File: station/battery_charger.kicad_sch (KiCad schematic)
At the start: 1 part, among them J8 Conn_01x04

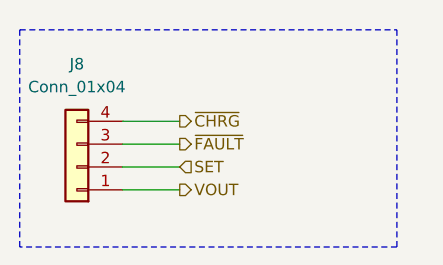
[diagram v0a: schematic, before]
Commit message: Signed-off-by: Scott Perkins <whatisbyandby@gmail.com>
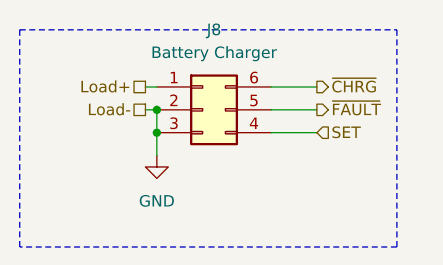
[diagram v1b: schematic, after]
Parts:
- removed J8: Conn_01x04, Connector_PinSocket_2.54mm:PinSocket_1x04_P2.54mm_Horizontal, symbol Connector_Generic:Conn_01x04
- added J8: Battery Charger, Connector_PinSocket_2.54mm:PinSocket_2x03_P2.54mm_Vertical, symbol Connector_Generic:Conn_02x03_Counter_Clockwise
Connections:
- net SET: now also J8.4 (Pin_4)
- net ~{CHRG}: now also J8.6 (Pin_6)
- net ~{FAULT}: now also J8.5 (Pin_5)
- new net GND: J8.2 (Pin_2), J8.3 (Pin_3)
- new net Load+: J8.1 (Pin_1)
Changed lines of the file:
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@@
 	(generator_version "8.0")
 	(paper "A4")
-	(wire
-		(pts
-			(xy 109.22 91.44) (xy 115.57 91.44)
-		)
-		(stroke
-			(width 0)
-			(type default)
-		)
-	)
-	(wire
-		(pts
-			(xy 109.22 86.36) (xy 115.57 86.36)
-		)
-		(stroke
-			(width 0)
-			(type default)
-		)
-	)
-	(wire
-		(pts
-			(xy 109.22 88.9) (xy 115.57 88.9)
-		)
-		(stroke
-			(width 0)
-			(type default)
-		)
-	)
-	(wire
-		(pts
-			(xy 109.22 93.98) (xy 115.57 93.98)
+	(junction
+		(at 113.03 87.63)
+		(diameter 0)
+		(color 0 0 0 0)
+	)
+	(junction
+		(at 113.03 85.09)
+		(diameter 0)
+		(color 0 0 0 0)
+	)
+	(wire
+		(pts
+			(xy 125.73 87.63) (xy 130.81 87.63)
+		)
+		(stroke
+			(width 0)
+			(type default)
+		)
+	)
+	(wire
+		(pts
+			(xy 113.03 87.63) (xy 113.03 90.17)
+		)
+		(stroke
+			(width 0)
+			(type default)
+		)
+	)
+	(wire
+		(pts
+			(xy 111.76 85.09) (xy 113.03 85.09)
+		)
+		(stroke
+			(width 0)
+			(type default)
+		)
+	)
+	(wire
+		(pts
+			(xy 125.73 82.55) (xy 130.81 82.55)
+		)
+		(stroke
+			(width 0)
+			(type default)
+		)
+	)
+	(wire
+		(pts
+			(xy 125.73 85.09) (xy 130.81 85.09)
+		)
+		(stroke
+			(width 0)
+			(type default)
+		)
+	)
+	(wire
+		(pts
+			(xy 113.03 85.09) (xy 113.03 87.63)
+		)
+		(stroke
+			(width 0)
+			(type default)
+		)
+	)
+	(wire
+		(pts
+			(xy 111.76 82.55) (xy 113.03 82.55)
 		)
 		(stroke
@@
 	(hierarchical_label "~{CHRG}"
 		(shape output)
-		(at 115.57 86.36 0)
+		(at 130.81 82.55 0)
 		(fields_autoplaced yes)
 		(effects
@@
 	(hierarchical_label "~{FAULT}"
 		(shape output)
-		(at 115.57 88.9 0)
+		(at 130.81 85.09 0)
 		(fields_autoplaced yes)
 		(effects
@@
 	(hierarchical_label "SET"
 		(shape input)
-		(at 115.57 91.44 0)
+		(at 130.81 87.63 0)
 		(fields_autoplaced yes)
 		(effects
@@
 		)
 	)
-	(hierarchical_label "VOUT"
-		(shape output)
-		(at 115.57 93.98 0)
-		(fields_autoplaced yes)
-		(effects
-			(font
-				(size 1.27 1.27)
-			)
-			(justify left)
+	(hierarchical_label "Load+"
+		(shape passive)
+		(at 111.76 82.55 180)
+		(fields_autoplaced yes)
+		(effects
+			(font
+				(size 1.27 1.27)
+			)
+			(justify right)
+		)
+	)
+	(hierarchical_label "Load-"
+		(shape passive)
+		(at 111.76 85.09 180)
+		(fields_autoplaced yes)
+		(effects
+			(font
+				(size 1.27 1.27)
+			)
+			(justify right)
 		)
 	)
 	(symbol
-		(lib_id "Connector_Generic:Conn_01x04")
-		(at 104.14 91.44 180)
+		(lib_id "power:GND")
+		(at 113.03 90.17 0)
 		(unit 1)
 		(exclude_from_sim no)
@@
 		(dnp no)
 		(fields_autoplaced yes)
+		(property "Reference" "#PWR024"
+			(at 113.03 96.52 0)
+			(effects
+				(font
+					(size 1.27 1.27)
+				)
+				(hide yes)
+			)
+		)
+		(property "Value" "GND"
+			(at 113.03 95.25 0)
+			(effects
+				(font
+					(size 1.27 1.27)
+				)
+			)
+		)
+		(property "Footprint" ""
+			(at 113.03 90.17 0)
+			(effects
+				(font
+					(size 1.27 1.27)
+				)
+				(hide yes)
+			)
+		)
+		(property "Datasheet" ""
+			(at 113.03 90.17 0)
+			(effects
+				(font
+					(size 1.27 1.27)
+				)
+				(hide yes)
+			)
+		)
+		(property "Description" "Power symbol creates a global label with name \"GND\" , ground"
+			(at 113.03 90.17 0)
+			(effects
+				(font
+					(size 1.27 1.27)
+				)
+				(hide yes)
+			)
+		)
+		(pin "1"
+		)
+		(instances
+			(project "weather_station_pico"
+				(path "/8f1f45aa-e764-4c95-a223-c466cf9a95bf/42d4f7d6-4f97-4f29-a0cd-bf4a015f7c0a"
+					(reference "#PWR024")
+					(unit 1)
+				)
+			)
+		)
+	)
+	(symbol
+		(lib_id "Connector_Generic:Conn_02x03_Counter_Clockwise")
+		(at 118.11 85.09 0)
+		(unit 1)
+		(exclude_from_sim no)
+		(in_bom yes)
+		(on_board yes)
+		(dnp no)
+		(fields_autoplaced yes)
 		(property "Reference" "J8"
-			(at 104.14 80.01 0)
-			(effects
-				(font
-					(size 1.27 1.27)
-				)
-			)
-		)
-		(property "Value" "Conn_01x04"
-			(at 104.14 82.55 0)
-			(effects
-				(font
-					(size 1.27 1.27)
-				)
-			)
-		)
-		(property "Footprint" "Connector_PinSocket_2.54mm:PinSocket_1x04_P2.54mm_Horizontal"
-			(at 104.14 91.44 0)
+			(at 119.38 76.2 0)
+			(effects
+				(font
+					(size 1.27 1.27)
+				)
+			)
+		)
+		(property "Value" "Battery Charger"
+			(at 119.38 78.74 0)
+			(effects
+				(font
+					(size 1.27 1.27)
+				)
+			)
+		)
+		(property "Footprint" "Connector_PinSocket_2.54mm:PinSocket_2x03_P2.54mm_Vertical"
+			(at 118.11 85.09 0)
 			(effects
 				(font
@@
 		)
 		(property "Datasheet" "~"
-			(at 104.14 91.44 0)
-			(effects
-				(font
-					(size 1.27 1.27)
-				)
-				(hide yes)
-			)
-		)
-		(property "Description" "Generic connector, single row, 01x04, script generated (kicad-library-utils/schlib/autogen/connector/)"
-			(at 104.14 91.44 0)
-			(effects
-				(font
-					(size 1.27 1.27)
-				)
-				(hide yes)
-			)
+			(at 118.11 85.09 0)
+			(effects
+				(font
+					(size 1.27 1.27)
+				)
+				(hide yes)
+			)
+		)
+		(property "Description" "Generic connector, double row, 02x03, counter clockwise pin numbering scheme (similar to DIP package numbering), script generated (kicad-library-utils/schlib/autogen/connector/)"
+			(at 118.11 85.09 0)
+			(effects
+				(font
+					(size 1.27 1.27)
+				)
+				(hide yes)
+			)
+		)
+		(pin "2"
+		)
+		(pin "5"
+		)
+		(pin "6"
+		)
+		(pin "1"
 		)
 		(pin "3"
 		)
-		(pin "2"
-		)
 		(pin "4"
 		)
-		(pin "1"
-		)
 		(instances
